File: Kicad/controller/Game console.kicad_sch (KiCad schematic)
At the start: 6 parts, among them SW1 SW_Push, SW2 SW_Push, SW3 SW_Push

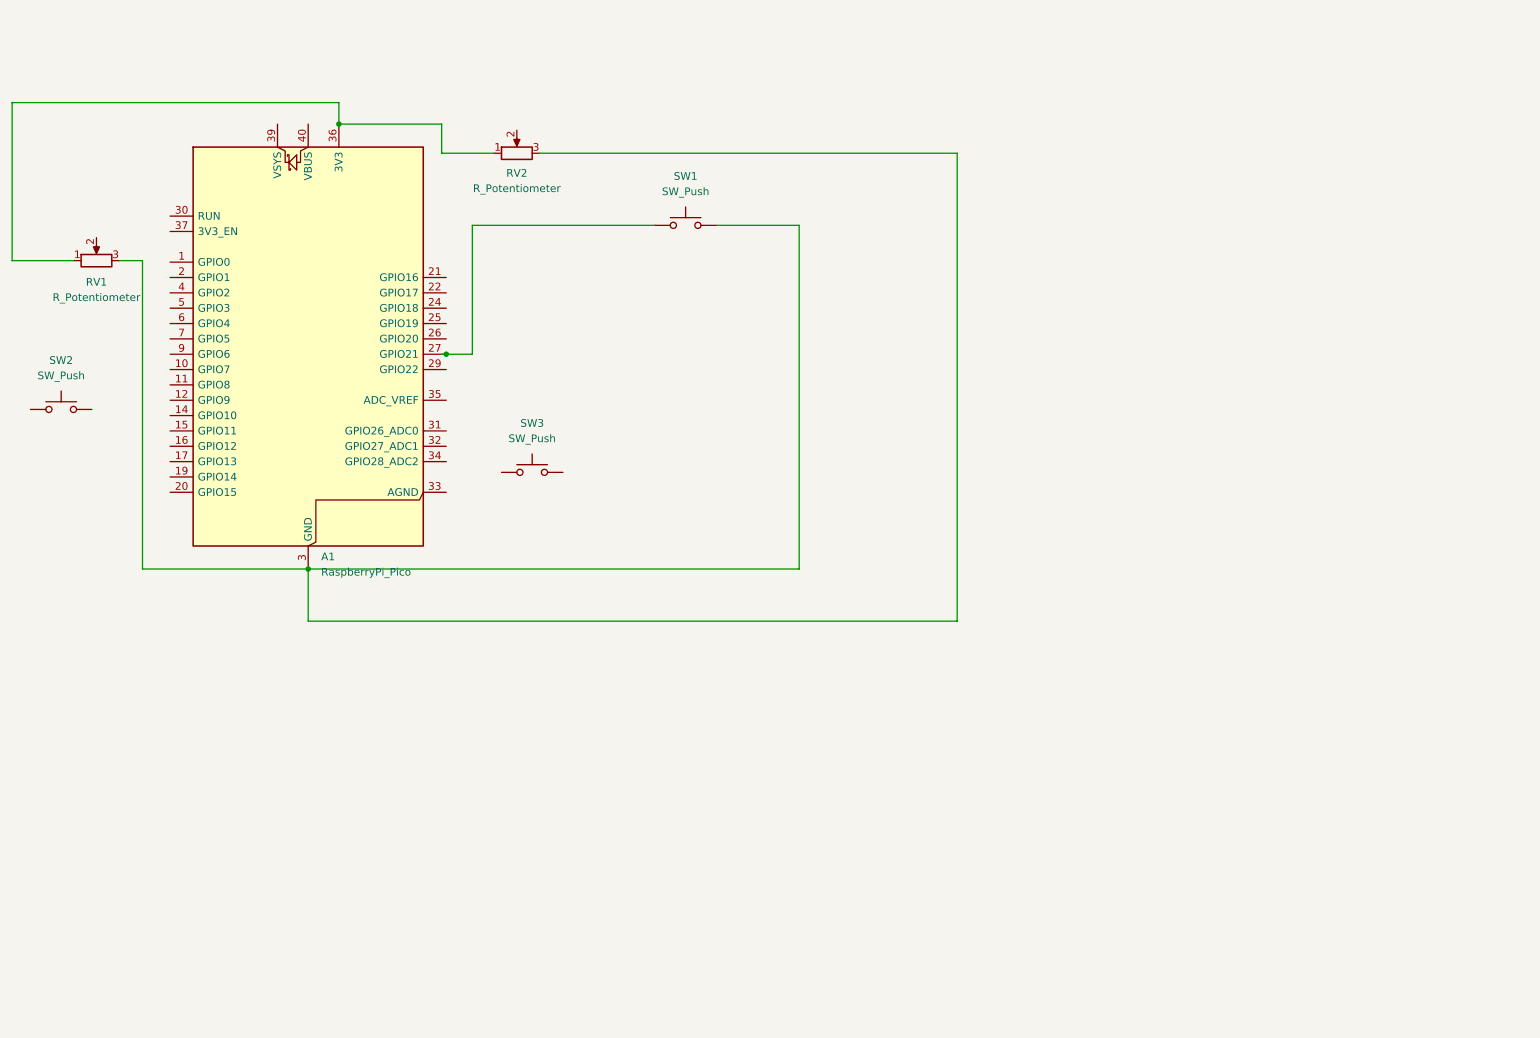
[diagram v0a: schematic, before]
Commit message: writing firmware codee
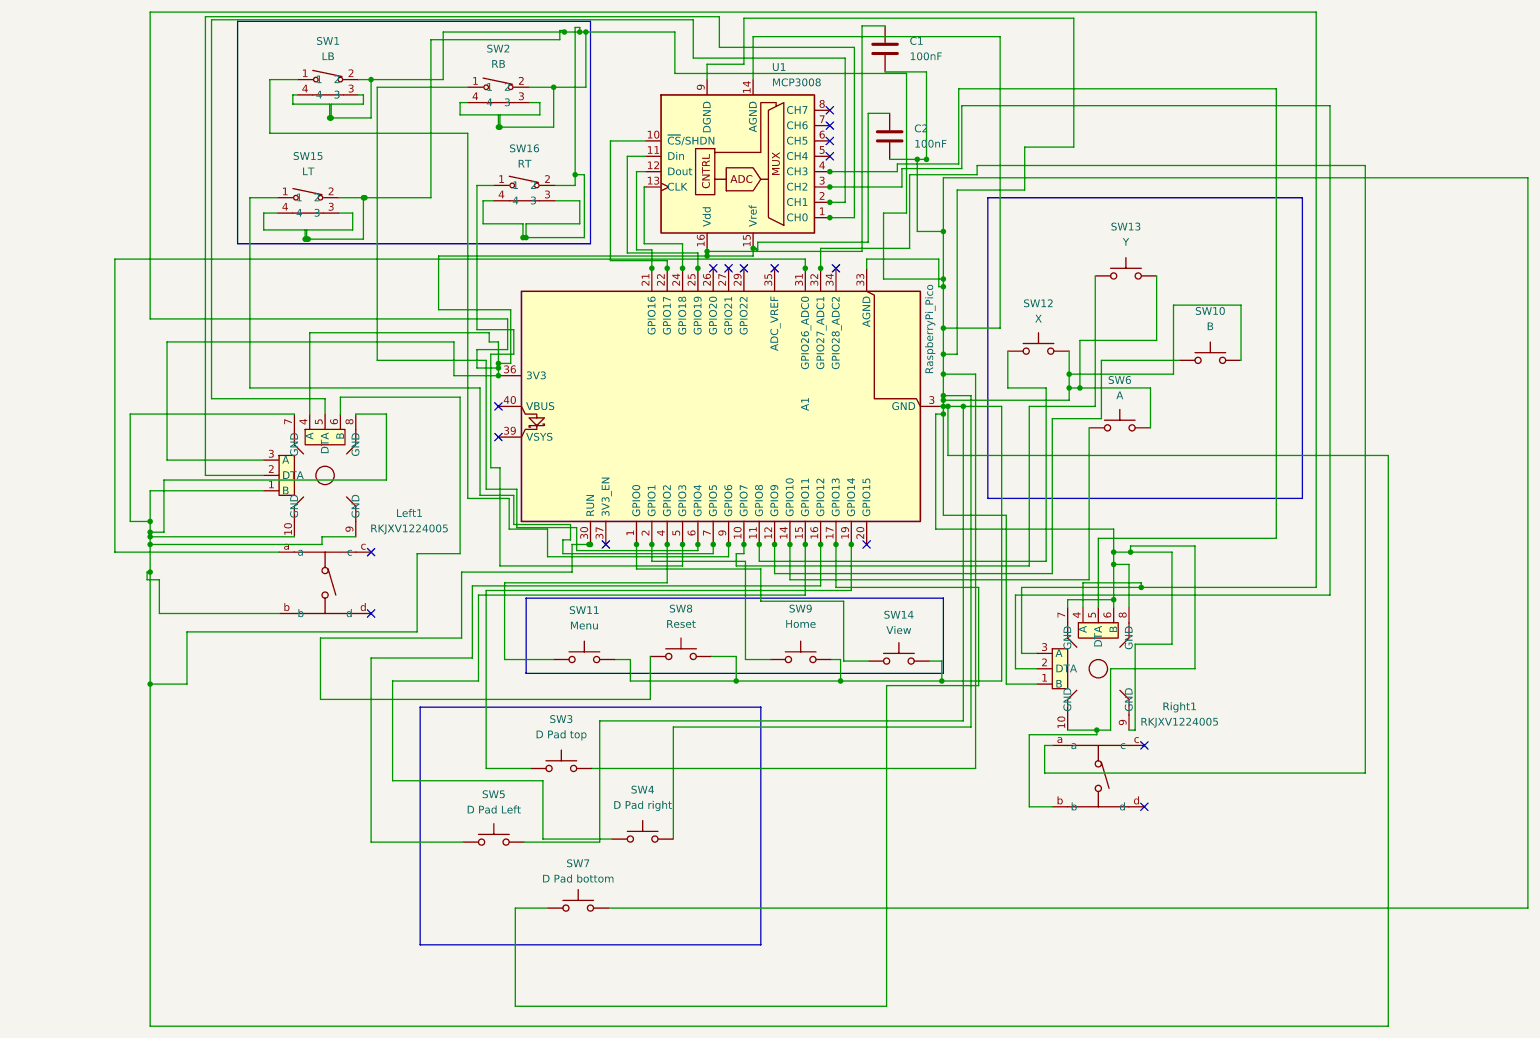
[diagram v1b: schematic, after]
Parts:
- removed RV1, RV2: R_Potentiometer, symbol Device:R_Potentiometer
- removed SW1, SW2: SW_Push, symbol Switch:SW_Push
- added C1, C2: 100nF, Capacitor_THT:C_Disc_D5.0mm_W2.5mm_P2.50mm, symbol Device:C
- added Left1, Right1: RKJXV1224005, easyeda2kicad:SW-TH_RKJXV1224005, symbol easyeda2kicad:RKJXV1224005
- added SW1: LB, easyeda2kicad:SW-TH_TC-1102N-C-DL-B, symbol easyeda2kicad:TC-1102N-C-DL-B
- added SW10: B, Button_Switch_THT:SW_PUSH_6mm_H5mm, symbol Switch:SW_Push
- added SW11: Menu, Button_Switch_THT:SW_PUSH_6mm_H5mm, symbol Switch:SW_Push
- added SW12: X, Button_Switch_THT:SW_PUSH_6mm_H5mm, symbol Switch:SW_Push
- added SW13: Y, Button_Switch_THT:SW_PUSH_6mm_H5mm, symbol Switch:SW_Push
- added SW14: View, Button_Switch_THT:SW_PUSH_6mm_H5mm, symbol Switch:SW_Push
- added SW15: LT, easyeda2kicad:SW-TH_TC-1102N-C-DL-B, symbol easyeda2kicad:TC-1102N-C-DL-B
- added SW16: RT, easyeda2kicad:SW-TH_TC-1102N-C-DL-B, symbol easyeda2kicad:TC-1102N-C-DL-B
- added SW2: RB, easyeda2kicad:SW-TH_TC-1102N-C-DL-B, symbol easyeda2kicad:TC-1102N-C-DL-B
- added SW4: D Pad right, Button_Switch_THT:SW_PUSH_6mm_H5mm, symbol Switch:SW_Push
- added SW5: D Pad Left, Button_Switch_THT:SW_PUSH_6mm_H5mm, symbol Switch:SW_Push
- added SW6: A, Button_Switch_THT:SW_PUSH_6mm_H5mm, symbol Switch:SW_Push
- added SW7: D Pad bottom, Button_Switch_THT:SW_PUSH_6mm_H5mm, symbol Switch:SW_Push
- added SW8: Reset, Button_Switch_THT:SW_PUSH_6mm_H5mm, symbol Switch:SW_Push
- added SW9: Home, Button_Switch_THT:SW_PUSH_6mm_H5mm, symbol Switch:SW_Push
- added U1: MCP3008, Package_DIP:DIP-16_W7.62mm, symbol Analog_ADC:MCP3008
- SW3: value SW_Push -> D Pad top; footprint (none) -> Button_Switch_THT:SW_PUSH_6mm_H5mm
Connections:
- net at SW3.1: now also A1.19 (GPIO14)
- net at SW3.2: now also A1.13 (GND), A1.18 (GND), A1.23 (GND), A1.28 (GND), A1.3 (GND), A1.33 (AGND), A1.38 (GND), A1.8 (GND), C1.2, C2.2, Left1.1 (B), Left1.10 (GND), Left1.6 (B), Left1.7 (GND), Left1.8 (GND), Left1.9 (GND), Left1.b, Right1.1 (B), Right1.10 (GND), Right1.6 (B), Right1.7 (GND), Right1.8 (GND), Right1.9 (GND), Right1.b, SW1.2, SW1.3, SW1.4, SW10.2, SW11.2, SW12.2, SW13.2, SW14.2, SW15.2, SW15.3, SW15.4, SW16.2, SW16.3, SW16.4, SW2.2, SW2.3, SW2.4, SW4.2, SW5.2, SW6.2, SW7.2, SW8.2, SW9.2, U1.14 (AGND), U1.9 (DGND)
- net at A1.36 (3V3): now also C1.1, C2.1, Left1.3 (A), Left1.4 (A), Right1.3 (A), Right1.4 (A), U1.15 (Vref), U1.16 (Vdd)
- net at A1.1 (GPIO0): now also SW14.1
- net at A1.10 (GPIO7): now also SW13.1
- net at A1.11 (GPIO8): now also SW12.1
- net at A1.12 (GPIO9): now also SW10.1
- net at A1.14 (GPIO10): now also SW6.1
- net at A1.15 (GPIO11): now also SW4.1
- net at A1.16 (GPIO12): now also SW5.1
- net at A1.17 (GPIO13): now also SW7.1
- net at A1.2 (GPIO1): now also SW9.1
- net at A1.21 (GPIO16): now also U1.12 (Dout)
- net at A1.22 (GPIO17): now also U1.10 (~{CS}/SHDN)
- net at A1.24 (GPIO18): now also U1.13 (CLK)
- net at A1.25 (GPIO19): now also U1.11 (Din)
- net at A1.30 (RUN): now also SW8.1
- net at A1.31 (GPIO26_ADC0): now also Left1.a
- net at A1.32 (GPIO27_ADC1): now also Right1.a
- net at A1.4 (GPIO2): now also SW11.1
- net at A1.5 (GPIO3): now also SW16.1
- net at A1.6 (GPIO4): now also SW2.1
- net at A1.7 (GPIO5): now also SW15.1
- net at A1.9 (GPIO6): now also SW1.1
- new net: Left1.2 (DTA), U1.1 (CH0)
- new net: Left1.5 (DTA), U1.2 (CH1)
- new net: Right1.2 (DTA), U1.3 (CH2)
- new net: Right1.5 (DTA), U1.4 (CH3)
- no-connect marks 0 -> 17
